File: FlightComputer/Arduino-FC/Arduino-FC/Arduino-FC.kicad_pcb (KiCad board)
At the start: 2 copper layers, 130 x 86.9 mm, 30 parts, among them J1 Conn_01x04, J2 Conn_01x08, J3 Conn_01x06, J4 Conn_01x03, J5 Screw_Terminal_01x02, J6 Conn_01x02, J7 Conn_01x02, U1 NRF24L01_Breakout

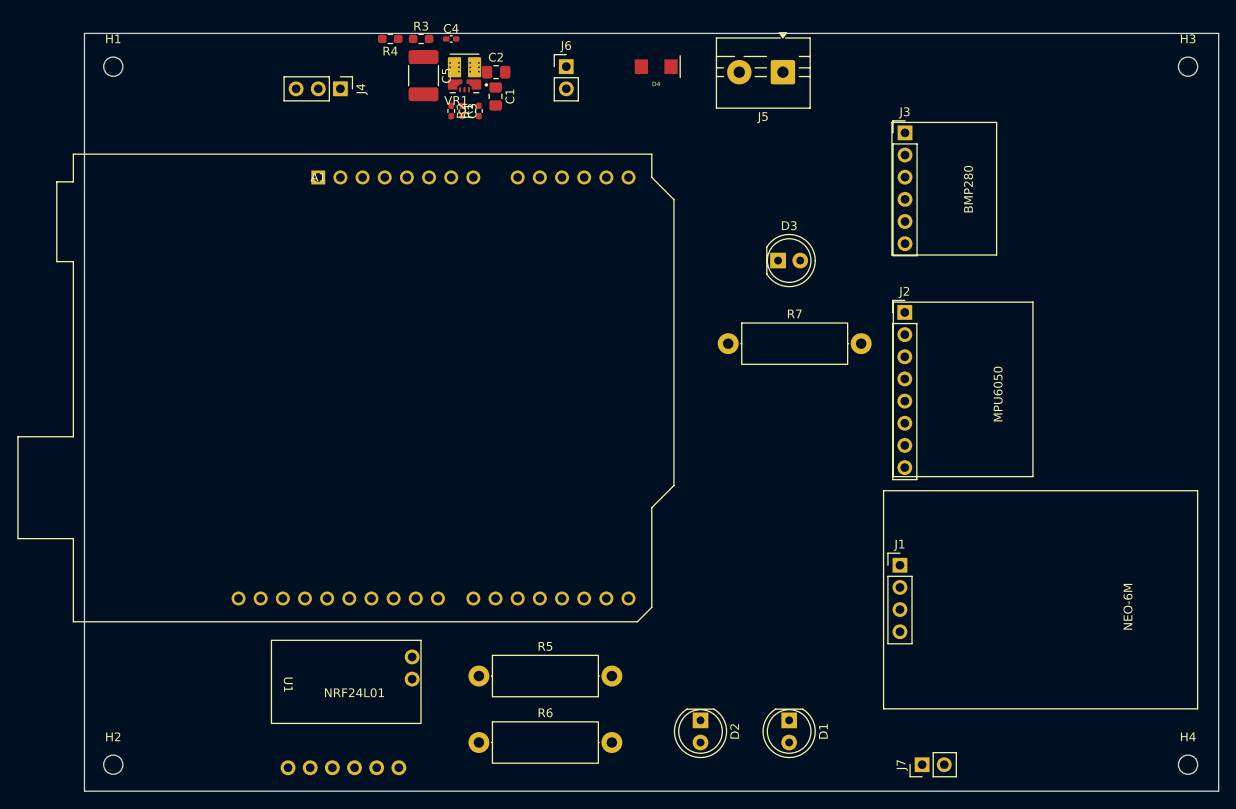
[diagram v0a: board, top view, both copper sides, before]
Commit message: Design Constraints
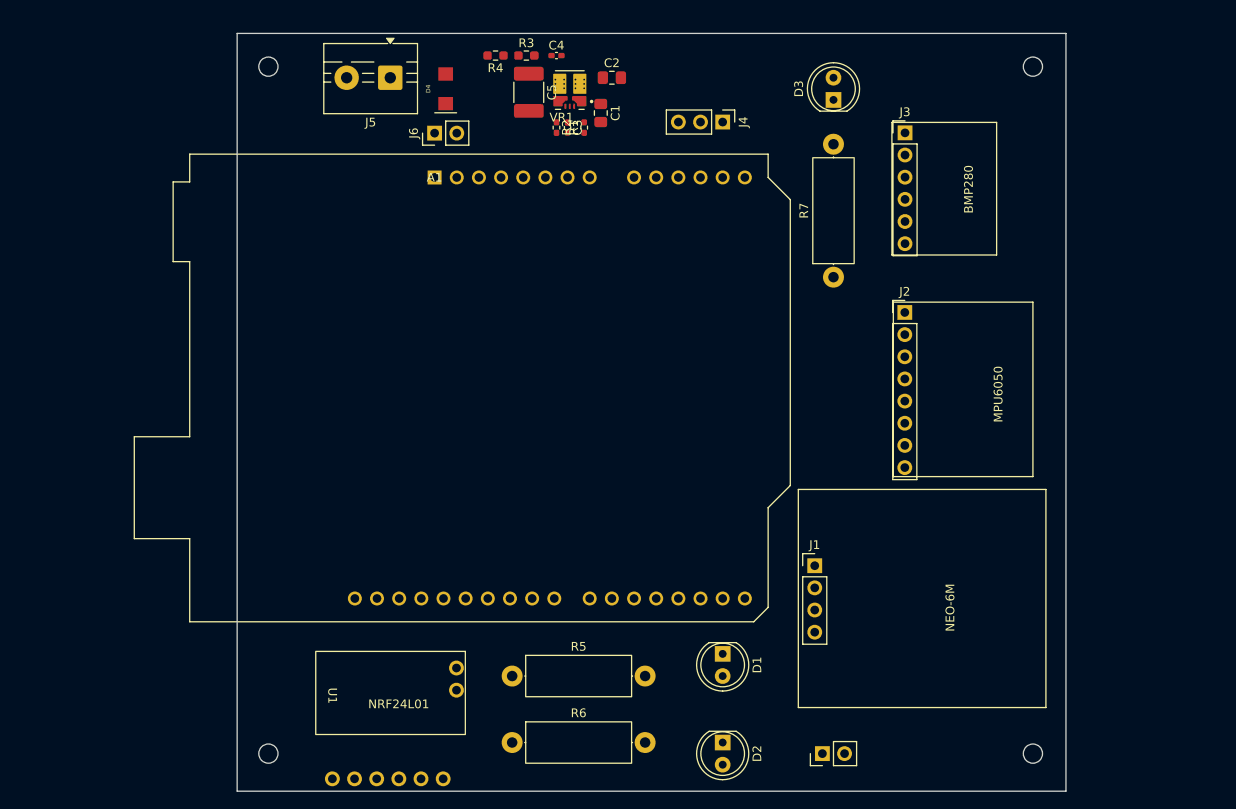
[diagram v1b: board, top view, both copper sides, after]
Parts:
- moved J5 45.0 mm to (127.0, 48.3)
- moved J4 44.0 mm to (165.1, 53.3)
- moved D4 24.3 mm to (133.3, 49.5), turned to 90 degrees
- moved D3 19.5 mm to (177.8, 50.8), turned to 90 degrees
- moved H2 17.8 mm to (113.0, 125.7)
- moved H4 17.8 mm to (200.7, 125.7)
- moved H1 17.8 mm to (113.0, 47.0)
- moved H3 17.8 mm to (200.7, 47.0)
- moved J6 16.9 mm to (132.1, 54.6), turned to 90 degrees
- moved R7 14.3 mm to (177.8, 71.1), turned to 90 degrees
- moved A1 13.3 mm to (132.1, 59.7)
- moved C2 13.3 mm to (152.4, 48.3)
- moved C1 12.2 mm to (151.1, 52.3)
- moved C3 12.2 mm to (147.3, 54.0)
- moved C4 12.2 mm to (146.1, 45.7)
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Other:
- board size 130 x 86.9 mm -> 95 x 86.9 mm
